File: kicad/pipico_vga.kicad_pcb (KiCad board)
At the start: 2 copper layers, 37 x 67 mm, 48 parts, among them J1 Conn_01x15, J2 DB15_Male_HighDensity_Mountin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, U1 Pico, U2 74LVC162244ADGVJ

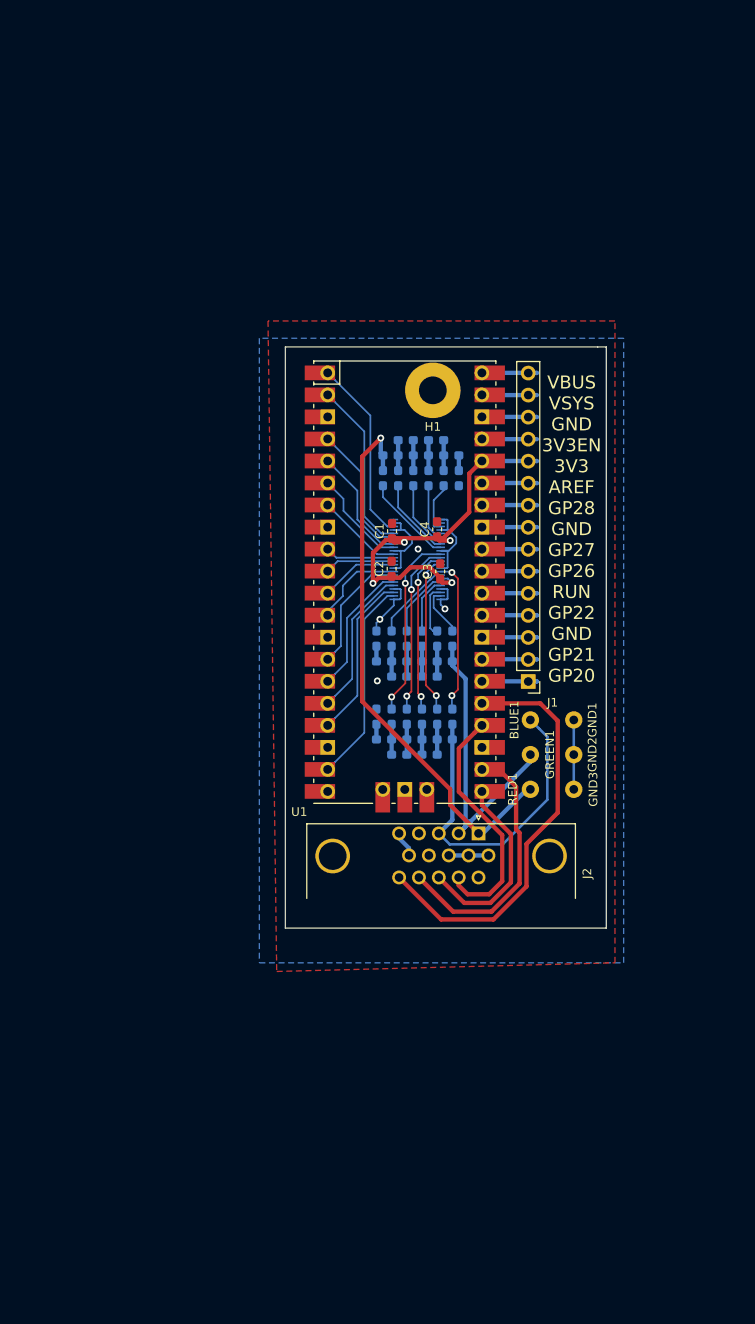
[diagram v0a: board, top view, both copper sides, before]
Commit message: Rev3 pcb and initial SW
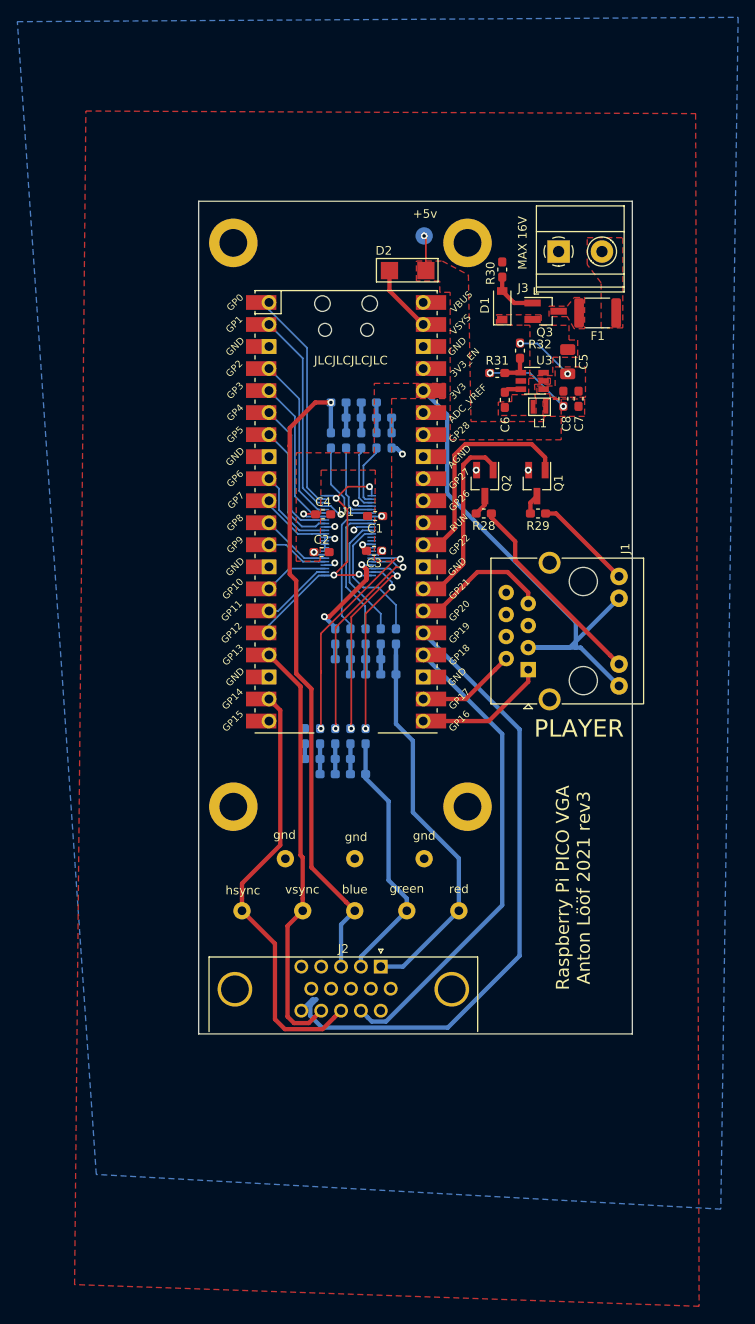
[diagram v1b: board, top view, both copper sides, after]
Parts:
- removed BLUE1, GREEN1, RED1: TestPoint, TestPoint:TestPoint_THTPad_D2.0mm_Drill1.0mm
- removed R33: 270, Resistor_SMD:R_0603_1608Metric_Pad1.05x0.95mm_HandSolder
- added C5: 10u 18v, Capacitor_SMD:C_1206_3216Metric, F.Cu at (153.6, 65.7)
- added C6: 100n, Capacitor_SMD:C_0603_1608Metric_Pad1.05x0.95mm_HandSolder, F.Cu at (146.3, 70.1)
- added C7: 22u 5v, Capacitor_SMD:C_0603_1608Metric_Pad1.05x0.95mm_HandSolder, F.Cu at (154.8, 70.0)
- added C8: 22u 5v, Capacitor_SMD:C_0603_1608Metric_Pad1.05x0.95mm_HandSolder, F.Cu at (153.1, 70.0)
- added D1: BZT52C5V1+, Diode_SMD:D_SOD-123, F.Cu at (146.0, 59.2)
- added D2: RSX301L-30TE25, good_things:SOD-106, F.Cu at (135.1, 55.2)
- added F1: MC36232, Fuse:Fuse_1812_4532Metric, F.Cu at (157.0, 60.1)
- added H2: MountingHole_Pad, MountingHole:MountingHole_3.2mm_M3_DIN965_Pad, B.Cu at (115.0, 52.0)
- added H3: MountingHole_Pad, MountingHole:MountingHole_3.2mm_M3_DIN965_Pad, B.Cu at (115.0, 117.0)
- added H4: MountingHole_Pad, MountingHole:MountingHole_3.2mm_M3_DIN965_Pad, B.Cu at (142.0, 52.0)
- added J3: power, TerminalBlock_Phoenix:TerminalBlock_Phoenix_MKDS-1,5-2_1x02_P5.00mm_Horizontal, F.Cu at (152.5, 53.0)
- added L1: 2u2, good_things:smd_inductor_0806_2016metric, F.Cu at (150.3, 70.9)
- added Q1: 2N7002P, Package_TO_SOT_SMD:SOT-23_Handsoldering, F.Cu at (150.0, 79.7)
- added Q2: 2N7002P, Package_TO_SOT_SMD:SOT-23_Handsoldering, F.Cu at (144.0, 79.7)
- added Q3: CPH3350-TL-W, Package_TO_SOT_SMD:SOT-23_Handsoldering, F.Cu at (151.0, 59.9)
- added TP1: red, TestPoint:TestPoint_THTPad_D2.0mm_Drill1.0mm, B.Cu at (141.0, 129.0)
- added TP2: green, TestPoint:TestPoint_THTPad_D2.0mm_Drill1.0mm, B.Cu at (135.0, 129.0)
- added TP3: blue, TestPoint:TestPoint_THTPad_D2.0mm_Drill1.0mm, B.Cu at (129.0, 129.0)
- added TP4: hsync, TestPoint:TestPoint_THTPad_D2.0mm_Drill1.0mm, B.Cu at (116.0, 129.0)
- added TP5: vsync, TestPoint:TestPoint_THTPad_D2.0mm_Drill1.0mm, B.Cu at (123.0, 129.0)
- added TP6: 5v, TestPoint:TestPoint_Pad_D2.0mm, B.Cu at (137.0, 51.2)
- added U3: AP62250, Package_TO_SOT_SMD:TSOT-23-6, F.Cu at (149.5, 67.9)
- H1: footprint MountingHole:MountingHole_3.2mm_M3_Pad -> MountingHole:MountingHole_3.2mm_M3_DIN965_Pad; moved to B.Cu
- J1: value Conn_01x15 -> RJ45_LED_Shielded; footprint Connector_PinHeader_2.54mm:PinHeader_1x15_P2.54mm_Vertical -> Connector_RJ:RJ45_BEL_SS74301-00x_Vertical
- J2: footprint random_stuff:DSUB-15-HDEX15SNT -> good_things:DSUB-15-HDEX15SNT
- R10, R11, R19, R20, R21, R22: value 270 -> 536
- R15, R16, R17, R24, R25, R26, R27, R6: value 536 -> 270
- R28: value 536 -> 1k; moved to F.Cu
- R29: value 270 -> 1k; moved to F.Cu
- R30, R32: value 270 -> 10k; moved to F.Cu
- R31: value 270 -> 52k3; moved to F.Cu
- moved R30 57.2 mm to (146.0, 55.1), turned to 90 degrees
- moved H1 48.2 mm to (142.0, 117.0), turned to 0 degrees
- moved R32 47.7 mm to (148.1, 64.4), turned to 90 degrees
- moved R31 43.3 mm to (145.4, 67.0), turned to 0 degrees
- moved R18 38.3 mm to (129.4, 113.2), turned to 180 degrees
- moved R16 35.1 mm to (125.9, 113.2), turned to 180 degrees
- moved R15 34.4 mm to (124.1, 111.5), turned to 180 degrees
- moved GND3 34.2 mm to (121.0, 123.0)
- moved R12 33.0 mm to (126.8, 108.9), turned to 90 degrees
- moved R17 32.7 mm to (127.6, 111.5), turned to 180 degrees
- moved R13 31.6 mm to (128.5, 108.9), turned to 90 degrees
- moved R29 31.5 mm to (150.1, 83.2)
- moved R9 31.1 mm to (127.1, 70.4), turned to 0 degrees
- moved R14 30.6 mm to (130.2, 108.9), turned to 90 degrees
- moved R8 30.3 mm to (128.9, 72.2), turned to 0 degrees
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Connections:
- J1 pad 1: Net-(J1-Pad1) -> tx
- J1 pad 10: Net-(J1-Pad10) -> +3V3
- J1 pad 11: +3V3 -> Net-(J1-Pad11)
- J1 pad 12: Net-(J1-Pad12) -> +3V3
- J1 pad 2: Net-(J1-Pad2) -> rx
- J1 pad 3: GND -> +3V3
- J1 pad 4: Net-(J1-Pad4) -> (no net)
- J1 pad 5: Net-(J1-Pad5) -> (no net)
- J1 pad 6: Net-(J1-Pad6) -> (no net)
- J1 pad 7: Net-(J1-Pad7) -> connected
- R10 pad 2: Net-(R10-Pad2) -> GND
- R11 pad 1: /green -> Net-(R11-Pad1)
- R11 pad 2: Net-(R10-Pad1) -> /g0
- R12 pad 2: GND -> /g1
- R13 pad 2: /r0 -> /g2
- R14 pad 1: Net-(R14-Pad1) -> /green
- R14 pad 2: /r1 -> /g3
- R15 pad 1: Net-(R15-Pad1) -> Net-(R11-Pad1)
- R15 pad 2: /r2 -> Net-(R10-Pad1)
- R16 pad 1: Net-(R16-Pad1) -> Net-(R12-Pad1)
- R16 pad 2: /r3 -> Net-(R11-Pad1)
- R17 pad 1: /red -> Net-(R13-Pad1)
- R17 pad 2: /r4 -> Net-(R12-Pad1)
- R18 pad 1: Net-(R13-Pad1) -> /green
- R18 pad 2: Net-(R12-Pad1) -> Net-(R13-Pad1)
- R19 pad 1: Net-(R14-Pad1) -> Net-(R19-Pad1)
- R19 pad 2: Net-(R13-Pad1) -> GND
- R2 pad 2: /g0 -> /b0
- R20 pad 1: Net-(R15-Pad1) -> Net-(R20-Pad1)
- R20 pad 2: Net-(R14-Pad1) -> /r0
- R21 pad 1: Net-(R16-Pad1) -> Net-(R21-Pad1)
- R21 pad 2: Net-(R15-Pad1) -> /r1
- R22 pad 1: /red -> Net-(R22-Pad1)
- R22 pad 2: Net-(R16-Pad1) -> /r2
- R23 pad 1: Net-(R23-Pad1) -> /red
- R23 pad 2: GND -> /r3
- R24 pad 1: Net-(R24-Pad1) -> Net-(R20-Pad1)
- R24 pad 2: /b0 -> Net-(R19-Pad1)
- R25 pad 1: Net-(R25-Pad1) -> Net-(R21-Pad1)
- R25 pad 2: /b1 -> Net-(R20-Pad1)
- R26 pad 1: Net-(R26-Pad1) -> Net-(R22-Pad1)
- R26 pad 2: /b2 -> Net-(R21-Pad1)
- R27 pad 1: Net-(R27-Pad1) -> /red
- R27 pad 2: /b3 -> Net-(R22-Pad1)
- R28 pad 1: /blue -> Net-(J1-Pad11)
- R28 pad 2: /b4 -> Net-(Q2-Pad3)
- R29 pad 1: Net-(R24-Pad1) -> Net-(J1-Pad9)
- R29 pad 2: Net-(R23-Pad1) -> Net-(Q1-Pad3)
- R3 pad 2: /g1 -> /b1
- R30 pad 1: Net-(R25-Pad1) -> Net-(D1-Pad2)
- R30 pad 2: Net-(R24-Pad1) -> GND
- R31 pad 1: Net-(R26-Pad1) -> +5V
- R31 pad 2: Net-(R25-Pad1) -> /vsys_fb
- R32 pad 1: Net-(R27-Pad1) -> /vsys_fb
- R32 pad 2: Net-(R26-Pad1) -> GND
- R4 pad 1: Net-(R10-Pad2) -> Net-(R4-Pad1)
- R4 pad 2: /g2 -> /b2
- R5 pad 1: Net-(R10-Pad1) -> /blue
- R5 pad 2: /g3 -> /b3
- R6 pad 1: /green -> Net-(R2-Pad1)
- R6 pad 2: /g4 -> Net-(R1-Pad1)
- R7 pad 1: Net-(R2-Pad1) -> Net-(R3-Pad1)
- R7 pad 2: Net-(R1-Pad1) -> Net-(R2-Pad1)
- R8 pad 1: Net-(R3-Pad1) -> Net-(R4-Pad1)
- R8 pad 2: Net-(R2-Pad1) -> Net-(R3-Pad1)
- R9 pad 1: Net-(R10-Pad2) -> /blue
- R9 pad 2: Net-(R3-Pad1) -> Net-(R4-Pad1)
- U1 pad 1: /gpio0 -> /pio_b0
- U1 pad 10: /gpio7 -> /pio_r3
- U1 pad 11: /gpio8 -> /pio_g0
- U1 pad 12: /gpio9 -> /pio_g1
- U1 pad 14: /gpio10 -> /pio_g2
- U1 pad 15: /gpio11 -> /pio_g3
- U1 pad 16: /gpio12 -> /rgb_oe
- U1 pad 17: /gpio13 -> /vsync
- U1 pad 19: /gpio14 -> /hsync
- U1 pad 2: /gpio1 -> /pio_b1
- U1 pad 21: /hsync -> tx
- U1 pad 22: /vsync -> rx
- U1 pad 26: Net-(J1-Pad1) -> connected
- U1 pad 27: Net-(J1-Pad2) -> /led1
- U1 pad 29: Net-(J1-Pad4) -> /led0
- U1 pad 30: Net-(J1-Pad5) -> Net-(U1-Pad30)
- U1 pad 31: Net-(J1-Pad6) -> Net-(U1-Pad31)
- U1 pad 32: Net-(J1-Pad7) -> Net-(U1-Pad32)
- U1 pad 34: Net-(J1-Pad9) -> Net-(U1-Pad34)
- U1 pad 35: Net-(J1-Pad10) -> Net-(U1-Pad35)
- U1 pad 37: Net-(J1-Pad12) -> Net-(U1-Pad37)
- U1 pad 39: Net-(J1-Pad14) -> Net-(D2-Pad1)
- U1 pad 4: /gpio2 -> /pio_b2
- U1 pad 40: Net-(J1-Pad15) -> Net-(U1-Pad40)
- U1 pad 5: /gpio3 -> /pio_b3
- U1 pad 6: /gpio4 -> /pio_r0
- U1 pad 7: /gpio5 -> /pio_r1
- U1 pad 9: /gpio6 -> /pio_r2
- U2 pad 1: GND -> /rgb_oe
- U2 pad 11: /gpio8 -> GND
- U2 pad 12: /gpio7 -> GND
- U2 pad 13: /gpio6 -> /pio_r3
- U2 pad 14: /gpio5 -> /pio_r2
- U2 pad 16: /gpio4 -> /pio_r1
- U2 pad 17: /gpio3 -> /pio_r0
- U2 pad 19: /gpio2 -> /pio_b3
- U2 pad 2: /gpio14 -> /pio_g3
- U2 pad 20: /gpio1 -> /pio_b2
- U2 pad 22: /gpio0 -> /pio_b1
- U2 pad 23: GND -> /pio_b0
- U2 pad 24: GND -> /rgb_oe
- U2 pad 25: GND -> /rgb_oe
- U2 pad 26: (no net) -> /b0
- U2 pad 27: /r0 -> /b1
- U2 pad 29: /r1 -> /b2
- U2 pad 3: /gpio13 -> /pio_g2
- U2 pad 30: /r2 -> /b3
- U2 pad 32: /r3 -> /r0
- U2 pad 33: /r4 -> /r1
- U2 pad 35: /b0 -> /r2
- U2 pad 36: /b1 -> /r3
- U2 pad 37: /b2 -> (no net)
- U2 pad 38: /b3 -> (no net)
- U2 pad 40: /b4 -> (no net)
- U2 pad 41: /g0 -> (no net)
- U2 pad 43: /g1 -> /g0
- U2 pad 44: /g2 -> /g1
- U2 pad 46: /g3 -> /g2
- U2 pad 47: /g4 -> /g3
- U2 pad 48: GND -> /rgb_oe
- U2 pad 5: /gpio12 -> /pio_g1
- U2 pad 6: /gpio11 -> /pio_g0
- U2 pad 8: /gpio10 -> GND
- U2 pad 9: /gpio9 -> GND
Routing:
- net /blue: track 38.6 -> 75.4 mm, vias 0 -> 1
- net GND: track 67.5 -> 34.8 mm, vias 4 -> 14
- net /rgb_oe: track 0.00 -> 32.2 mm, vias 0 -> 4
- net /hsync: track 22.4 -> 49.8 mm
- net /led0: track 0.00 -> 26.0 mm
- net /pio_b0: track 0.00 -> 25.8 mm
- net /vga_data: track 29.3 -> 55.0 mm
- net /vga_clk: track 50.2 -> 74.4 mm
- net /pio_b1: track 0.00 -> 23.7 mm
- net /gpio14: track 23.6 -> 0.00 mm
- net Net-(J1-Pad11): track 0.00 -> 23.5 mm
- net /led1: track 0.00 -> 22.0 mm
- net /gpio0: track 21.3 -> 0.00 mm
- net +3V3: track 49.9 -> 70.0 mm
- net /gpio1: track 20.0 -> 0.00 mm
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- added copper zone on F.Cu, net +3V3
- added copper zone on F.Cu, net +5V
- added copper zone on F.Cu, net /vin
- added copper zone on F.Cu, net /vin_raw
- added copper zone on F.Cu, net /vsys_sw
- added copper zone on F.Cu, net Net-(F1-Pad2)
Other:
- board size 37 x 67 mm -> 50 x 96 mm
- board text added: "+5v"
- board text added: "GND VIN"
- board text added: "JLCJLCJLCJLC"
- board text added: "MAX 16V"
- board text added: "PLAYER"
- board text added: "Raspberry Pi PICO VGA Anton Lööf 2021 rev3"
- board text added: "blue"
- board text added: "gnd"
- board text added: "green"
- board text added: "hsync"
- board text added: "red"
- board text added: "vsync"
- board text removed: "Anton Lööf 2021 REV3"
- board text removed: "Raspberry pi Pico VGA"
- board text removed: "VBUS VSYS GND 3V3EN 3V3 AREF GP28 GND GP27 GP26 RUN GP22 GND GP21 GP20"
